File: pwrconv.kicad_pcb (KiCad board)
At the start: 2 copper layers, 40 x 32 mm, 31 parts, among them J1 Power In, J2 Power Out, U1 TPS5430DDA, U2 TPS5430DDA, U3 TPS5430DDA

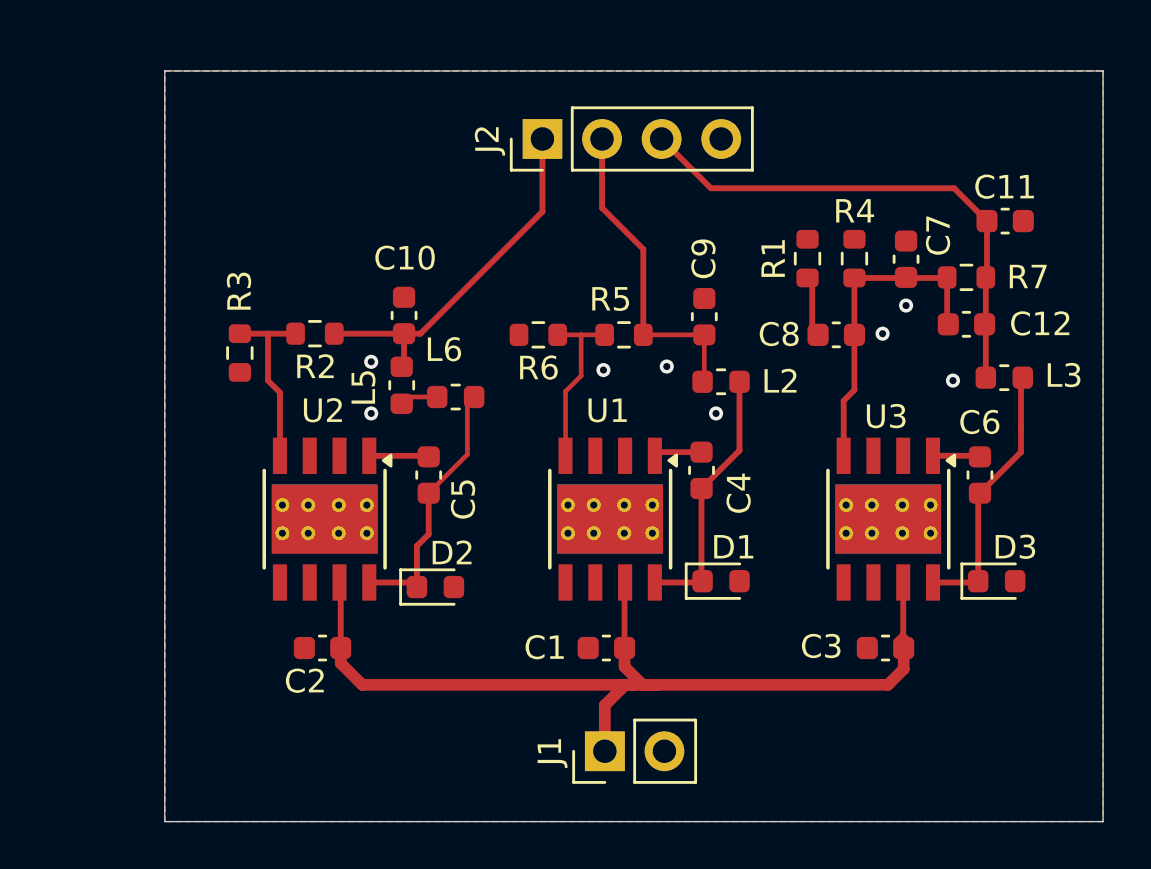
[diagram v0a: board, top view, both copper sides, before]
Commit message: Add files via upload
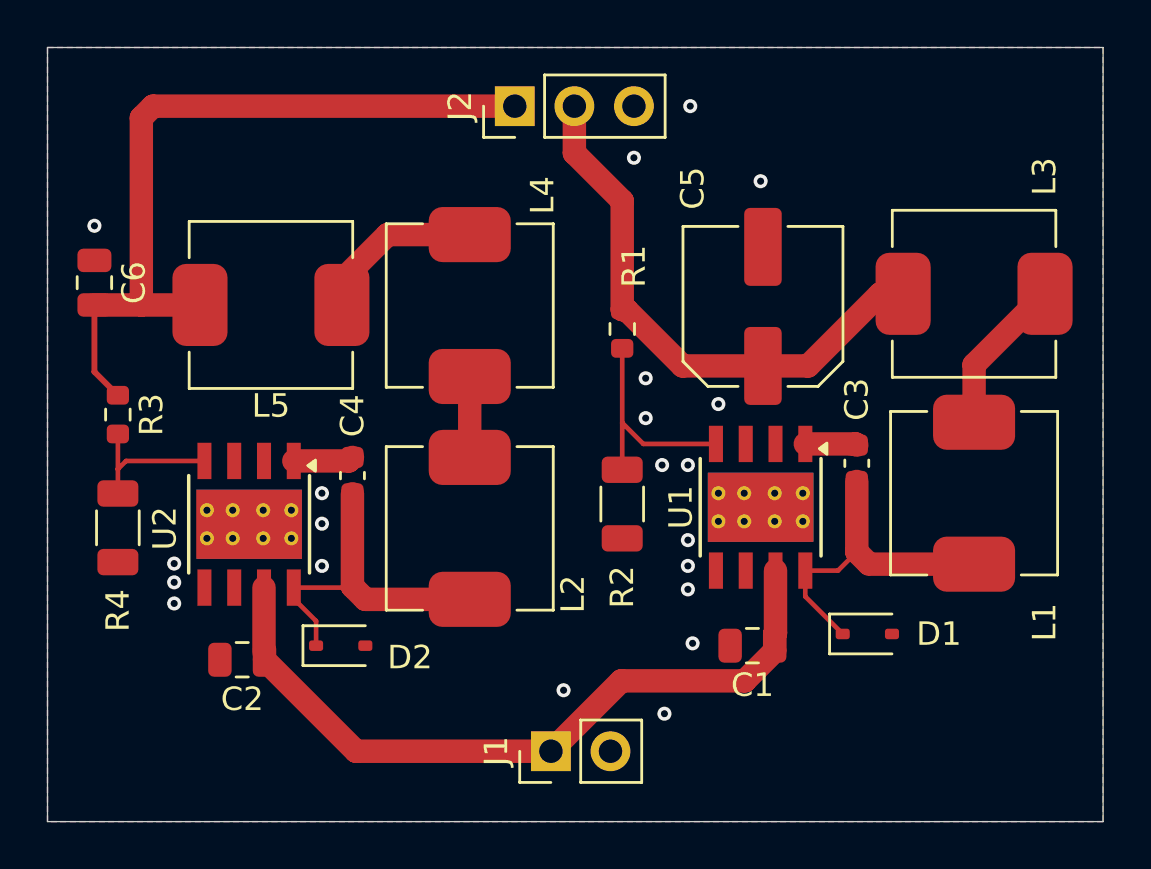
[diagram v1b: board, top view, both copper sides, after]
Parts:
- removed C10: 22u, Capacitor_SMD:C_0603_1608Metric
- removed C11: 100 μF, Capacitor_SMD:C_0603_1608Metric
- removed C12: 1500 pF, Capacitor_SMD:C_0603_1608Metric
- removed C7: 150 pF, Capacitor_SMD:C_0603_1608Metric
- removed C8: 0.1 μF, Capacitor_SMD:C_0603_1608Metric
- removed C9: 220uF, Capacitor_SMD:C_0603_1608Metric
- removed D3: D_Schottky, Diode_SMD:D_0603_1608Metric
- removed L6: 12u, Inductor_SMD:L_0603_1608Metric
- removed R5: 10K, Resistor_SMD:R_0603_1608Metric
- removed R6: 3.2K, Resistor_SMD:R_0603_1608Metric
- removed R7: 10 kΩ, Resistor_SMD:R_0603_1608Metric
- removed U3: TPS5430DDA, Package_SO:TI_SO-PowerPAD-8_ThermalVias
- added L1: 10uH, Inductor_SMD:L_Changjiang_FXL0630, F.Cu at (194.5, 66.0)
- added L4: 10uH, Inductor_SMD:L_Changjiang_FXL0630, F.Cu at (173.0, 58.0)
- C1: value 4.7 μF -> 4.7uF; footprint Capacitor_SMD:C_0603_1608Metric -> Capacitor_SMD:C_0805_2012Metric
- C2: value 10u -> 4.7uF; footprint Capacitor_SMD:C_0603_1608Metric -> Capacitor_SMD:C_0805_2012Metric
- C3: value 4.7uF -> 0.01 uF
- C4: value 0.01 uF -> 0.01uf
- C5: value 0.01uf -> 100uF; footprint Capacitor_SMD:C_0603_1608Metric -> Capacitor_SMD:C_Elec_6.3x7.7
- C6: value 0.01 μF -> 22u; footprint Capacitor_SMD:C_0603_1608Metric -> Capacitor_SMD:C_0805_2012Metric
- D1, D2: footprint Diode_SMD:D_0603_1608Metric -> Diode_SMD:D_SOD-323
- J2: footprint Connector_PinHeader_2.54mm:PinHeader_1x04_P2.54mm_Vertical -> Connector_PinHeader_2.54mm:PinHeader_1x03_P2.54mm_Vertical
- L2: value >=26 uH -> 10uH; footprint Inductor_SMD:L_0603_1608Metric -> Inductor_SMD:L_Changjiang_FXL0630
- L3: value 15 μH -> 10uH; footprint Inductor_SMD:L_0603_1608Metric -> Inductor_SMD:L_Changjiang_FXL0630
- L5: value 10u -> 10uH; footprint Inductor_SMD:L_0603_1608Metric -> Inductor_SMD:L_Changjiang_FXL0630
- R1: value 549 Ω -> 10K
- R2: value 10k -> 3.3K; footprint Resistor_SMD:R_0603_1608Metric -> Resistor_SMD:R_1206_3216Metric
- R3: value 1.13k -> 10k
- R4: value 5.9 kΩ -> 1k; footprint Resistor_SMD:R_0603_1608Metric -> Resistor_SMD:R_1206_3216Metric
- moved C6 38.6 mm to (157.0, 57.0)
- moved R4 33.4 mm to (158.0, 67.5), turned to -90 degrees
- moved C5 16.0 mm to (185.5, 58.0), turned to 90 degrees
- moved R2 15.0 mm to (179.5, 66.5), turned to -90 degrees
- moved C4 14.9 mm to (168.0, 65.2)
- moved L2 12.4 mm to (173.0, 67.5), turned to 90 degrees
- moved R1 8.45 mm to (179.5, 59.0), turned to -90 degrees
- moved C3 7.97 mm to (189.5, 64.7), turned to -90 degrees
- moved D1 6.63 mm to (189.9, 72.0)
- moved L5 6.54 mm to (164.5, 58.0), turned to 180 degrees
- moved U1 6.43 mm to (185.4, 66.6)
- moved C1 6.23 mm to (185.1, 72.5)
- moved R3 5.82 mm to (158.0, 62.6)
- moved D2 4.75 mm to (167.5, 72.5)
- moved L3 3.80 mm to (194.5, 57.5)
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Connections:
- C3 pad 1: +24V -> Net-(U1-BOOT)
- C3 pad 2: GND -> Net-(D1-K)
- C4 pad 1: Net-(U1-BOOT) -> Net-(U2-BOOT)
- C4 pad 2: Net-(D1-K) -> Net-(D2-K)
- C5 pad 1: Net-(U2-BOOT) -> +5V
- C5 pad 2: Net-(D2-K) -> GND
- C6 pad 1: Net-(U3-BOOT) -> GND
- C6 pad 2: Net-(D3-K) -> +12V
- J2 pad 3: +3.3V -> GND
- L2 pad 1: Net-(D1-K) -> Net-(D2-K)
- L2 pad 2: +5V -> Net-(L2-Pad2)
- L3 pad 1: Net-(D3-K) -> Net-(L1-Pad2)
- L3 pad 2: +3.3V -> +5V
- L5 pad 1: (no net) -> Net-(L4-Pad2)
- L5 pad 2: (no net) -> +12V
- R1 pad 1: Net-(C8-Pad2) -> +5V
- R1 pad 2: GND -> Net-(U1-VSENSE)
- R2 pad 1: +12V -> Net-(U1-VSENSE)
- R2 pad 2: Net-(U2-VSENSE) -> GND
- R3 pad 1: Net-(U2-VSENSE) -> +12V
- R3 pad 2: GND -> Net-(U2-VSENSE)
- R4 pad 1: Net-(U3-VSENSE) -> Net-(U2-VSENSE)
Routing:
- net +3.3V: track 22.0 -> 0.00 mm
- net +12V: track 15.5 -> 32.9 mm
- net Net-(U3-VSENSE): track 13.9 -> 0.00 mm
- net Net-(D3-K): track 11.4 -> 0.00 mm
- net +5V: track 13.3 -> 24.0 mm
- net +24V: track 41.0 -> 31.3 mm
- net Net-(L4-Pad2): track 0.00 -> 7.31 mm
- net Net-(L1-Pad2): track 0.00 -> 6.73 mm
- net Net-(D2-K): track 8.90 -> 14.6 mm
- net (no net): track 3.71 -> 0.00 mm
- net Net-(D1-K): track 11.1 -> 14.8 mm
- net Net-(L2-Pad2): track 0.00 -> 3.45 mm
- net Net-(C8-Pad2): track 2.61 -> 0.00 mm
- net Net-(U1-VSENSE): track 7.43 -> 9.55 mm
- net Net-(U3-BOOT): track 2.02 -> 0.00 mm
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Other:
- board size 40 x 32 mm -> 45 x 33 mm
